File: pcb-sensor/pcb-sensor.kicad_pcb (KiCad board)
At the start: 2 copper layers, 84 x 84 mm, 28 parts, among them J1 Conn_02x06_Counter_Clockwise, J2 Conn_01x03, J3 Conn_01x01, J4 Conn_01x05, J5 Conn_01x02, J6 Conn_01x03, J7 Conn_01x01, J8 Conn_01x01, U1 LM340MP, U2 SFH617A-1, U4 SFH617A-1

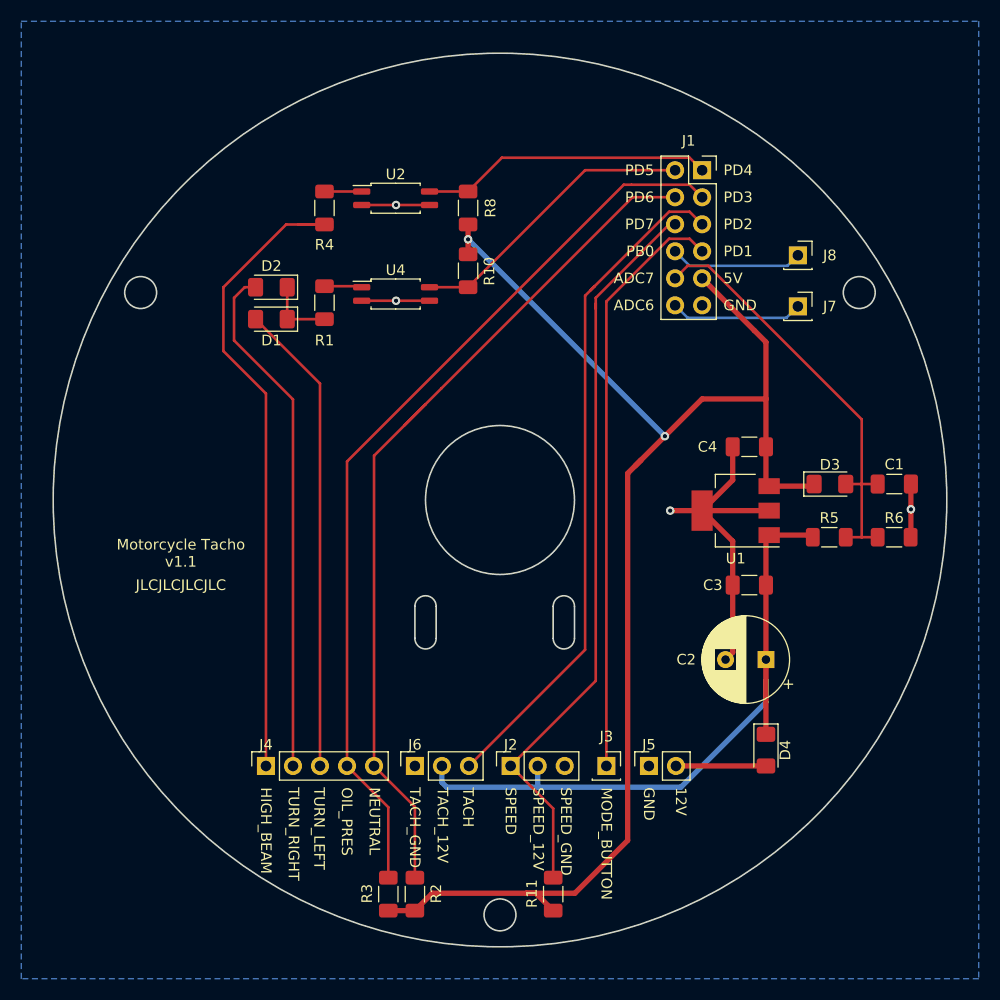
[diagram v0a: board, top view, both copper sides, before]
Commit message: v1.1
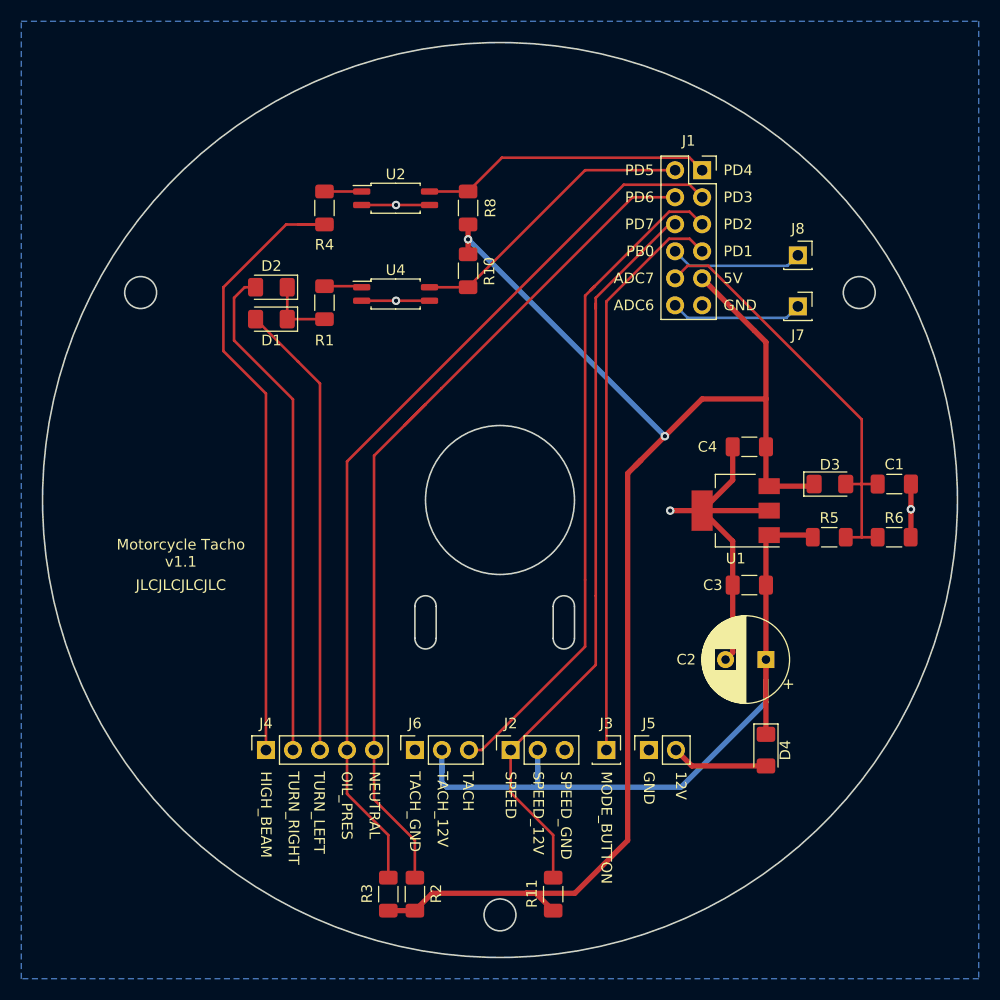
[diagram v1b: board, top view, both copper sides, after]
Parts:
- C1: value C -> 100n
- C2: value CP -> 100u
- D1, D2, D4: value 1N4148 -> 1N4001
- D3: value D -> 1N4001
- R11, R5: value R -> 10k
- R6: value R -> 4.7k
- moved J2 1.50 mm to (151.0, 123.5)
- moved J3 1.50 mm to (160.0, 123.5)
- moved J4 1.50 mm to (128.0, 123.5)
- moved J5 1.50 mm to (164.0, 123.5)
- moved J6 1.50 mm to (142.0, 123.5)
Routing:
- net +12V: track 66.4 -> 71.0 mm
- net /TURN_SIGNAL_LEFT: track 44.5 -> 43.0 mm
- net /TURN_SIGNAL_RIGHT: track 48.7 -> 47.2 mm
- net /MODE_BUTTON: track 55.6 -> 54.1 mm
- net /HIGH_BEAM: track 61.1 -> 59.6 mm
- net /PD2: track 64.0 -> 63.3 mm
- net Net-(D4-Pad2): track 8.46 -> 9.08 mm
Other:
- board size 84 x 84 mm -> 86 x 86 mm
